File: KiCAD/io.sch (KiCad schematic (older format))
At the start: 26 parts

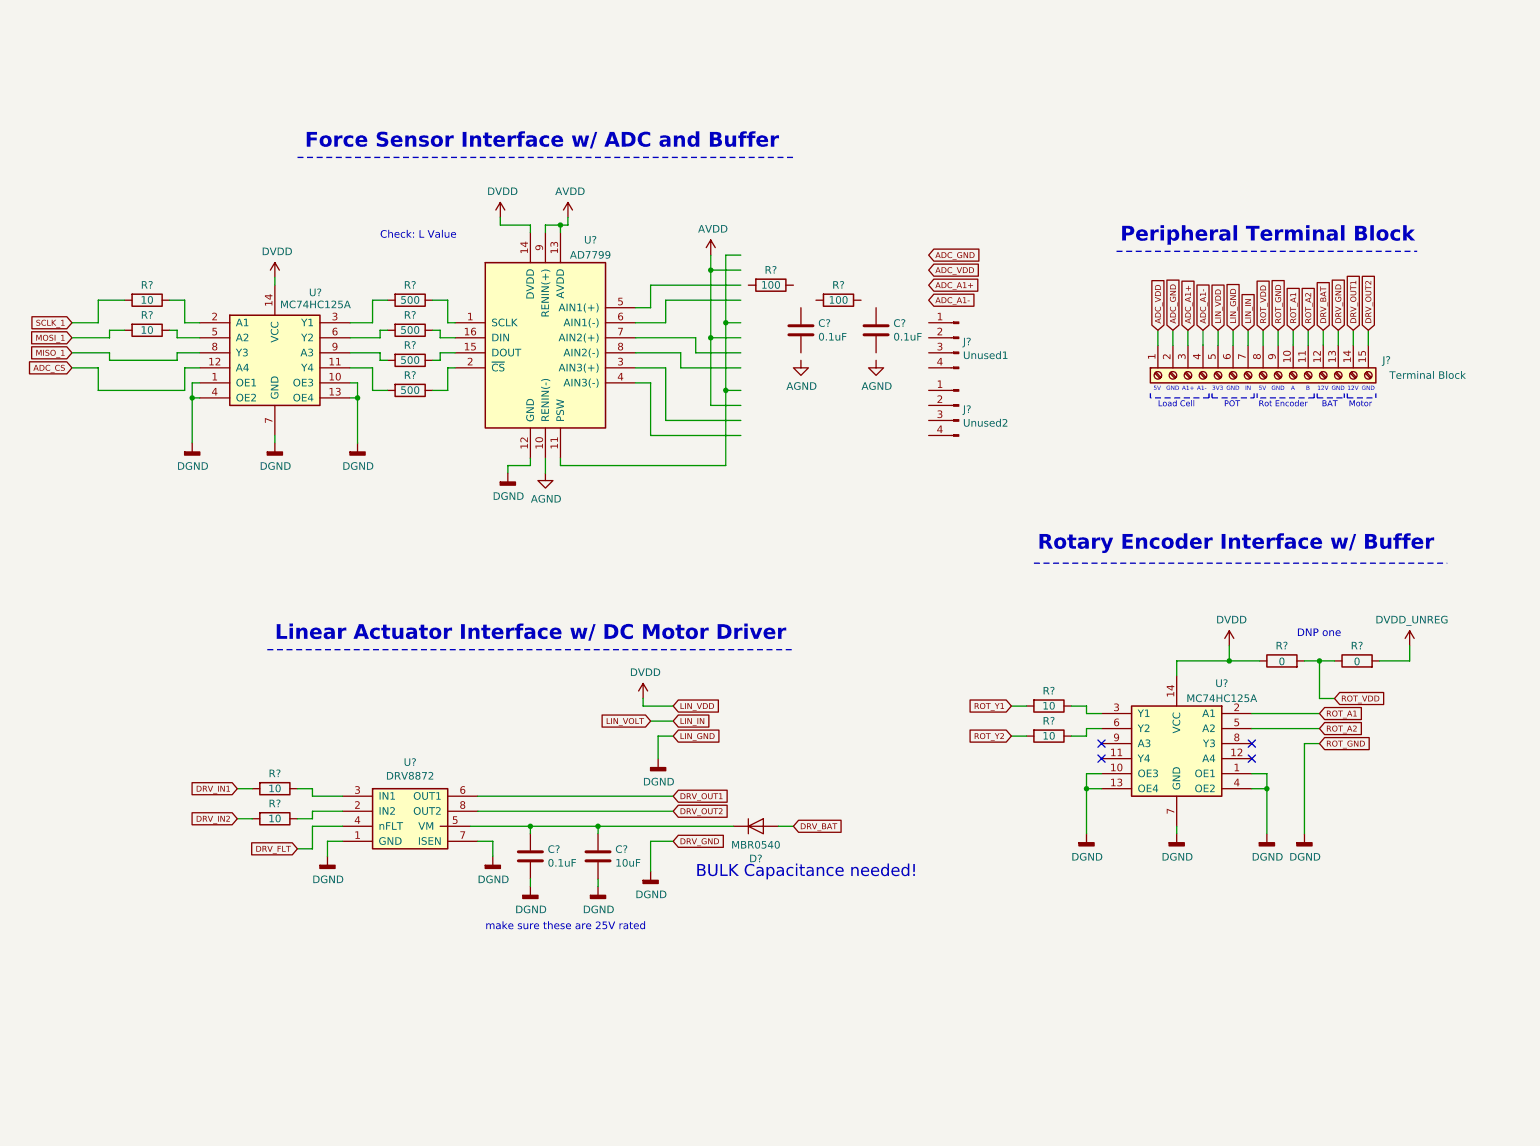
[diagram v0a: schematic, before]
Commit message: Decoupling caps & more
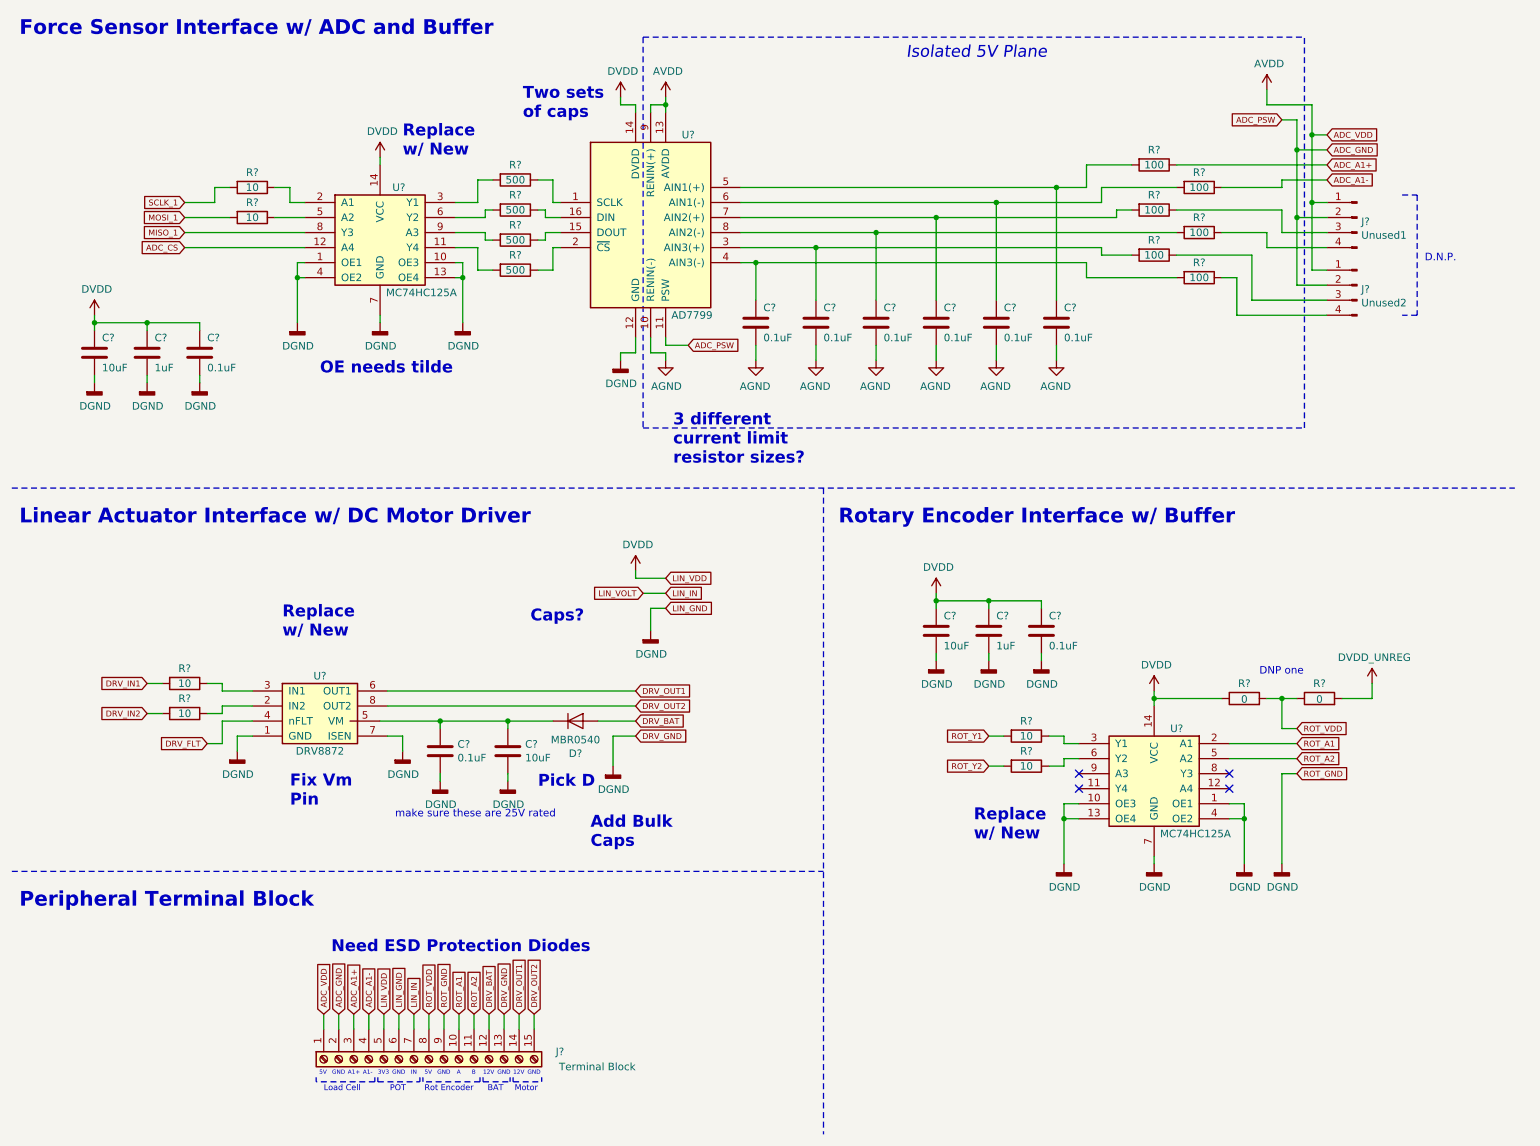
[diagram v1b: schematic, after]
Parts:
- removed C? (x2): 0.1uF, symbol Device:C
- removed J?: Unused1, symbol Connector:Conn_01x04_Male
- removed J?: Unused2, symbol Connector:Conn_01x04_Male
- removed R? (x2): 100, symbol Device:R
- added C? (x8): 0.1uF, symbol Device:C
- added C? (x2): 1uF, symbol Device:C
- added C? (x2): 10uF, symbol Device:C
- added J?: Unused1, symbol Connector:Conn_01x04_Male
- added J?: Unused2, symbol Connector:Conn_01x04_Male
- added R? (x6): 100, symbol Device:R
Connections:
- net labels added: ADC_PSW
- wire segments 178 -> 219
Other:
- note added: "3 different\ncurrent limit\nresistor sizes?"
- note added: "Add Bulk\nCaps"
- note added: "Caps?"
- note added: "D.N.P."
- note added: "Fix Vm\nPin"
- note added: "Isolated 5V Plane"
- note added: "Need ESD Protection Diodes"
- note added: "OE needs tilde"
- note added: "Pick D"
- note added: "Replace\nw/ New"
- note added: "Two sets\nof caps"
- note removed: "BULK Capacitance needed!"
- note removed: "Check: L Value"
- moved on the sheet: C?, D?, J?, R?, U?

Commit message: Before changing files
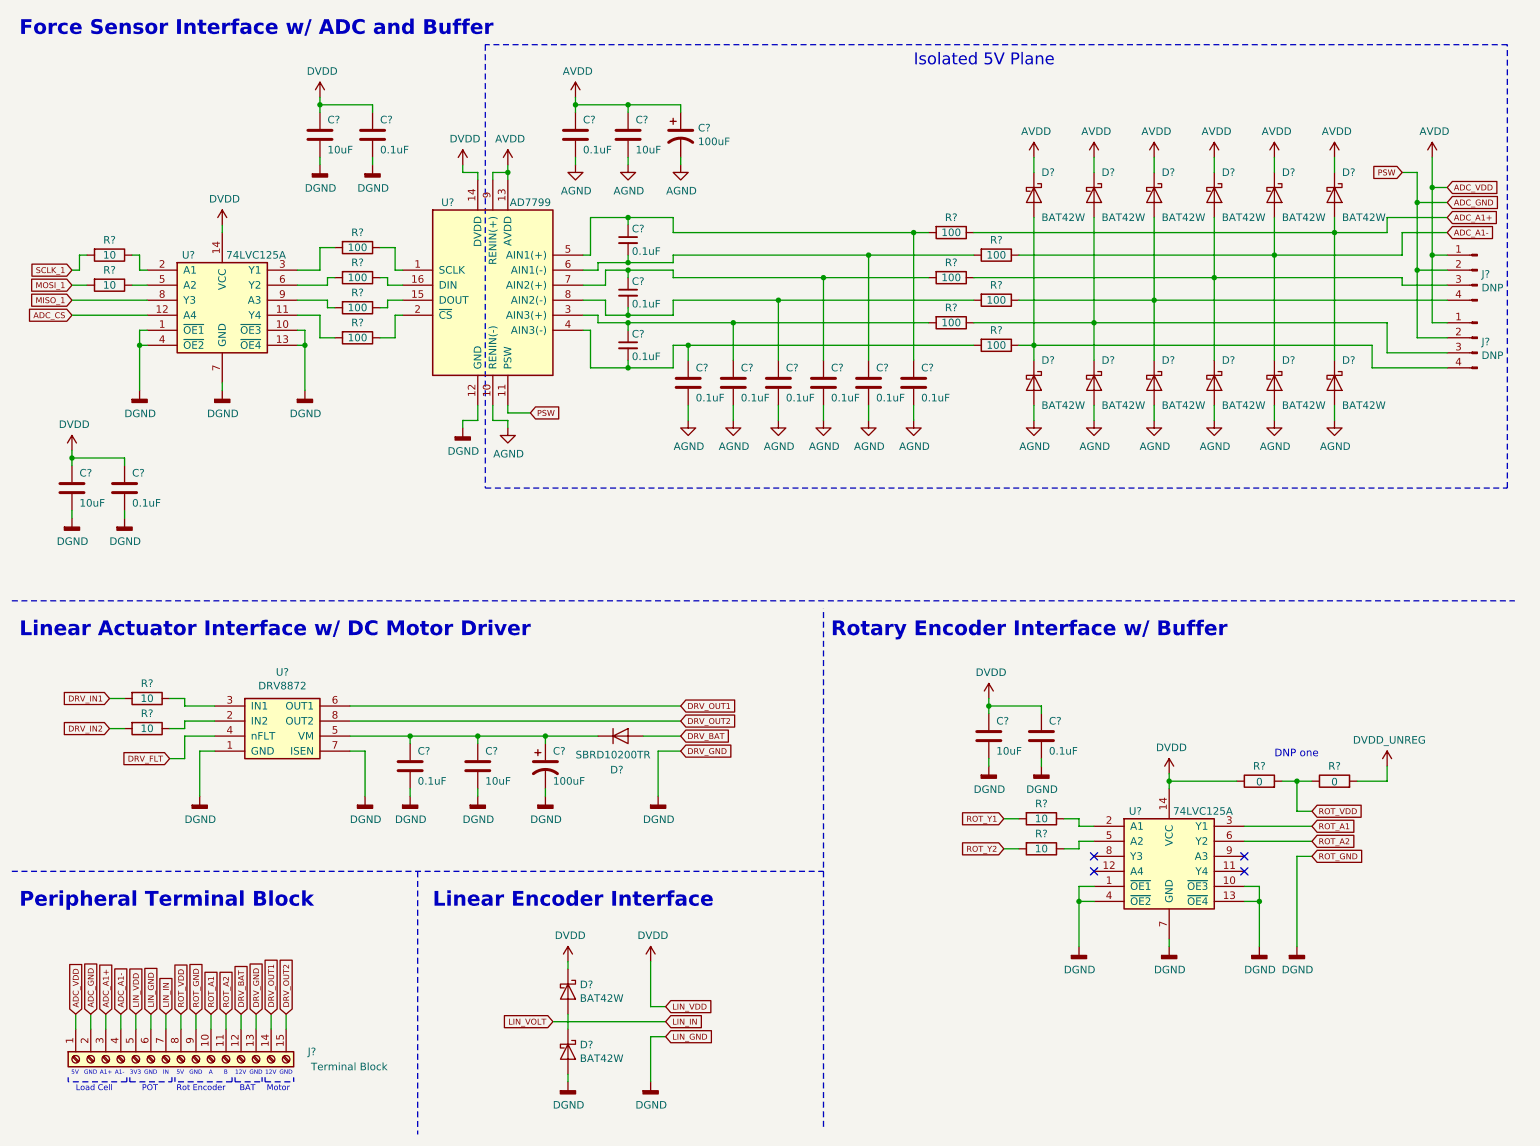
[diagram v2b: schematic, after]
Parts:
- removed C? (x2): 0.1uF, symbol Device:C
- removed C? (x2): 1uF, symbol Device:C
- removed C? (x2): 10uF, symbol Device:C
- removed U?: AD7799, symbol croptop_rev1-rescue:AD7799-croptop
- removed U? (x2): MC74HC125A, symbol croptop_rev1-rescue:MC74HC125A-croptop
- removed U?: DRV8872, symbol croptop_rev1-rescue:DRV8872-croptop
- added C? (x4): 0.1uF, symbol Device:C
- added C? (x4): 10uF, symbol Device:C
- added C? (x2): 100uF, symbol Device:CP1
- added C? (x3): 0.1uF, symbol Device:C_Small
- added D? (x14): BAT42W, symbol Device:D_Schottky
- added U?: AD7799, symbol CropTop:AD7799
- added U? (x2): 74LVC125A, symbol CropTop:74LVC125A
- added U?: DRV8872, symbol CropTop:DRV8872
- D?: value MBR0540 -> SBRD10200TR
- J?: value Unused1 -> DNP
- J?: value Unused2 -> DNP
- R? (x4): value 500 -> 100
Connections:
- net ADC_A1+: now also D?.1 (K), D?.2 (A)
- net ADC_A1-: now also D?.1 (K), D?.2 (A)
- net ADC_CS: now also U?.12 (A4)
- net ADC_GND: now also U?.11 (PSW)
- net AGND: now also C?.2, C?.2, C?.2, D?.2 (A), D?.2 (A), D?.2 (A), D?.2 (A), D?.2 (A), D?.2 (A), U?.10 (RENIN(-))
- net AVDD: now also C?.1, C?.1, C?.1, D?.1 (K), D?.1 (K), D?.1 (K), D?.1 (K), D?.1 (K), D?.1 (K), U?.13 (AVDD), U?.9 (RENIN(+))
- net DGND: now also C?.2, C?.2, C?.2, C?.2, C?.2, C?.2, C?.2, D?.2 (A), U?.1 (GND), U?.1 (~OE1), U?.1 (~OE1), U?.10 (~OE3), U?.10 (~OE3), U?.12 (GND), U?.13 (~OE4), U?.13 (~OE4), U?.4 (~OE2), U?.4 (~OE2), U?.7 (GND), U?.7 (GND), U?.7 (ISEN)
- net DRV_FLT: now also U?.4 (nFLT)
- net DRV_OUT1: now also U?.6 (OUT1)
- net DRV_OUT2: now also U?.8 (OUT2)
- net DVDD: now also C?.1, C?.1, C?.1, C?.1, C?.1, C?.1, D?.1 (K), U?.14 (DVDD), U?.14 (VCC), U?.14 (VCC)
- net MISO_1: now also U?.8 (Y3)
- net ROT_A1: now also U?.3 (Y1)
- net ROT_A2: now also U?.6 (Y2)
- net at C?.2, R?.2: now also C?.1, U?.5 (AIN1(+))
- net at C?.2, R?.2: now also C?.2, U?.6 (AIN1(-))
- net at J?.3 (Pin_3), R?.1: now also D?.1 (K), D?.2 (A) (x2)
- net at C?.2, R?.2: now also C?.1, U?.7 (AIN2(+))
- net at J?.4 (Pin_4), R?.1: now also D?.1 (K), D?.2 (A) (x2)
- net at C?.2, R?.2: now also C?.2, U?.8 (AIN2(-))
- net at C?.2, R?.2: now also C?.1, U?.3 (AIN3(+))
- net at C?.2, R?.2: now also C?.2, U?.4 (AIN3(-))
- net at R?.1: now also U?.1 (SCLK)
- net at R?.1: now also U?.15 (DOUT)
- net at R?.1: now also U?.16 (DIN)
- net at R?.1: now also U?.2 (~CS)
- net at R?.2: now also U?.11 (Y4)
- net at R?.1: now also U?.2 (A1) (x2)
- net at R?.2: now also U?.3 (Y1)
- net at R?.1: now also U?.5 (A2) (x2)
- net at R?.2: now also U?.6 (Y2)
- net at R?.2: now also U?.9 (A3)
- net at R?.1: now also U?.2 (IN2)
- net at R?.1: now also U?.3 (IN1)
- net at C?.1, C?.1, D?.1 (K): now also C?.1, U?.5 (VM)
- new net: D?.1 (K), D?.2 (A)
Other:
- note added: "Linear Encoder Interface"
- note removed: "3 different\ncurrent limit\nresistor sizes?"
- note removed: "Add Bulk\nCaps"
- note removed: "Caps?"
- note removed: "D.N.P."
- note removed: "Fix Vm\nPin"
- note removed: "Need ESD Protection Diodes"
- note removed: "OE needs tilde"
- note removed: "Pick D"
- note removed: "Replace\nw/ New"
- note removed: "Two sets\nof caps"
- note removed: "make sure these are 25V rated\n"
- moved on the sheet: C?, D?, J?, R?
